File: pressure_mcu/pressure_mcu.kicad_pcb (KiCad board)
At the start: 2 copper layers, 33.2 x 35 mm, 41 parts, among them J2 USB_B_Micro, J4 1, J5 2, J6 3, J7 4, J8 SWD JST PH, U2 AP2112K-3.3, U4 STM32H562RGT6, U7 TCA9548APWR, Y2 12MHz

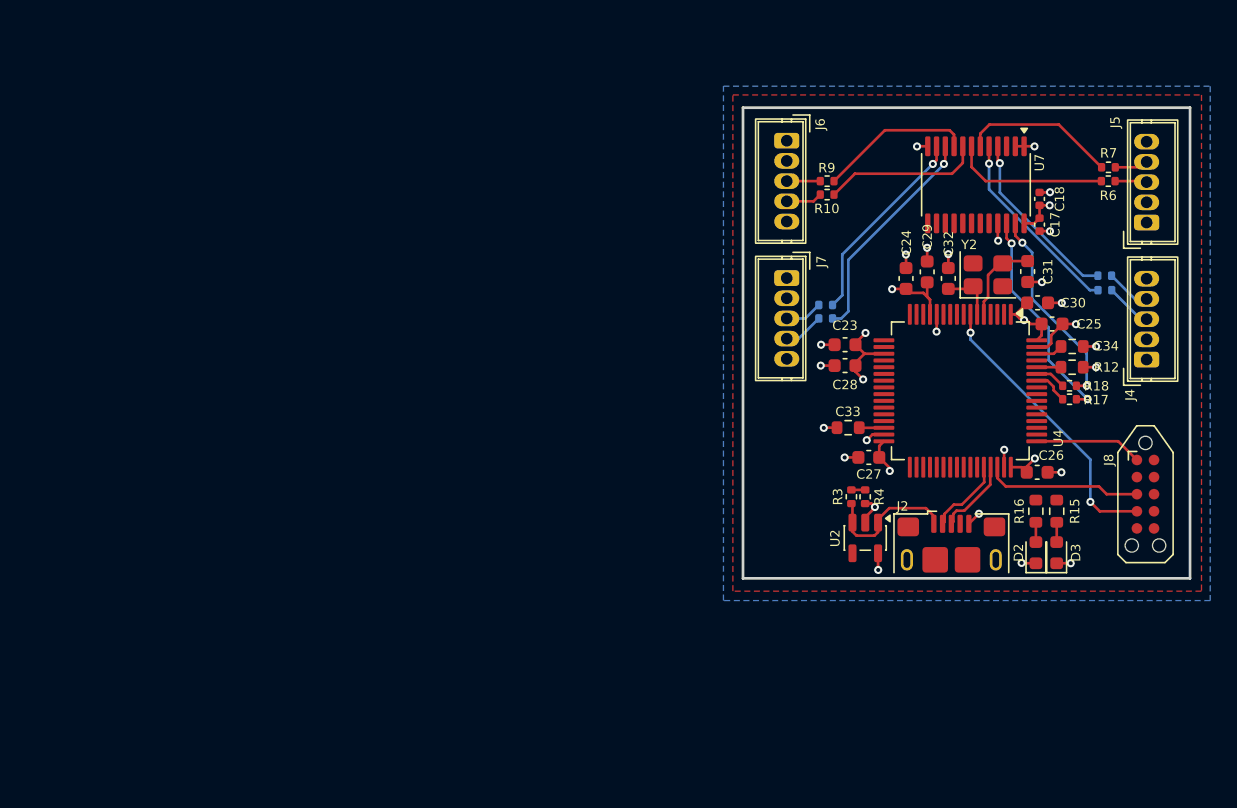
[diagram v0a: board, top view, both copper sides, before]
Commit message: ready for review
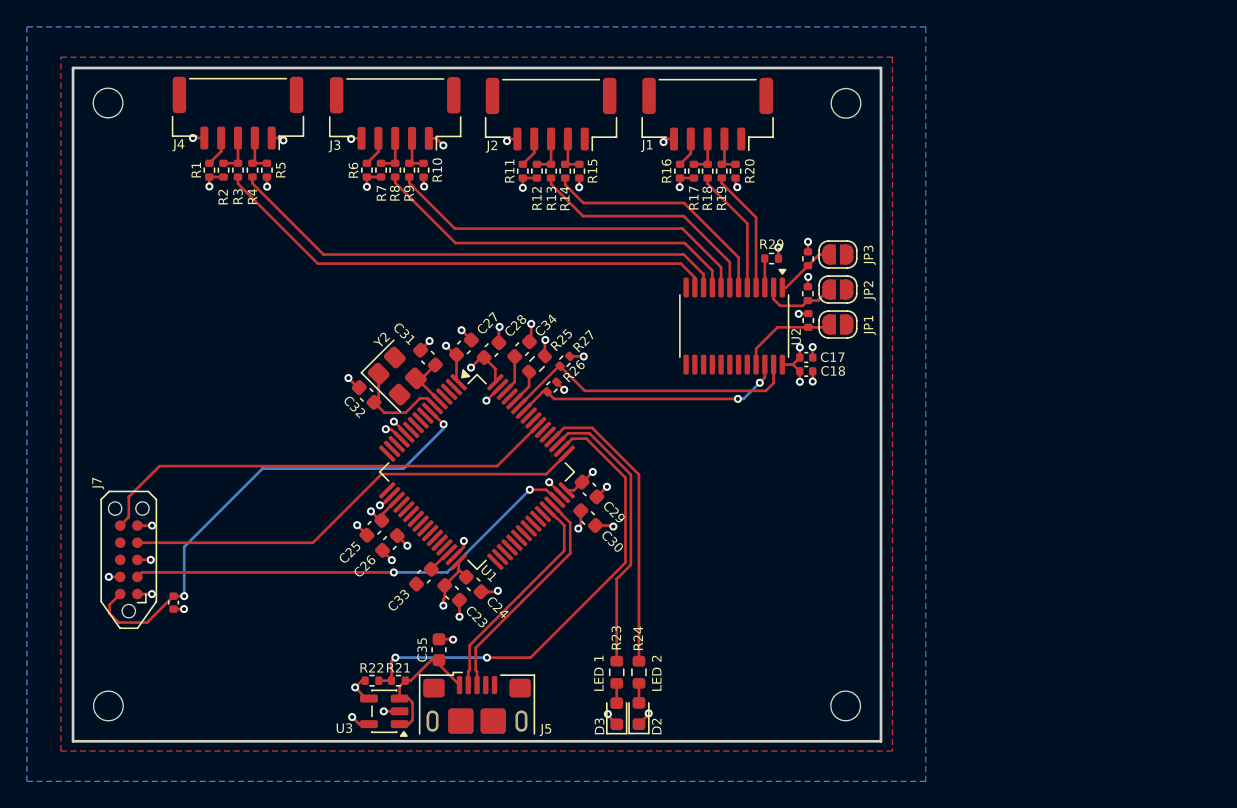
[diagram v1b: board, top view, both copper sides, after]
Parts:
- removed J6: 3, Connector_Wuerth:Wuerth_WR-WTB_64800511622_1x05_P1.50mm_Vertical
- removed J8: SWD JST PH, Connector:Tag-Connect_TC2050-IDC-NL_2x05_P1.27mm_Vertical_with_bottom_clip
- removed U4: STM32H562RGT6, Package_QFP:LQFP-64_10x10mm_P0.5mm
- removed U7: TCA9548APWR, Package_SO:TSSOP-24_4.4x7.8mm_P0.65mm
- added C35: 10uF, Capacitor_SMD:C_0603_1608Metric, F.Cu at (147.2, 118.2)
- added C36: 100nF, Capacitor_SMD:C_0402_1005Metric, F.Cu at (127.5, 114.7)
- added H1: MountingHole, MountingHole:MountingHole_2.2mm_M2, F.Cu at (122.6, 77.6)
- added H2: MountingHole, MountingHole:MountingHole_2.2mm_M2, F.Cu at (177.4, 77.6)
- added H3: MountingHole, MountingHole:MountingHole_2.2mm_M2, F.Cu at (122.6, 122.4)
- added H4: MountingHole, MountingHole:MountingHole_2.2mm_M2, F.Cu at (177.4, 122.4)
- added J1: 1, Connector_JST:JST_GH_SM05B-GHS-TB_1x05-1MP_P1.25mm_Horizontal, F.Cu at (167.1, 78.4)
- added J3: 3, Connector_JST:JST_GH_SM05B-GHS-TB_1x05-1MP_P1.25mm_Horizontal, F.Cu at (143.9, 78.4)
- added JP1: SolderJumper_2_Open, Jumper:SolderJumper-2_P1.3mm_Open_RoundedPad1.0x1.5mm, F.Cu at (176.8, 94.0)
- added JP2: SolderJumper_2_Open, Jumper:SolderJumper-2_P1.3mm_Open_RoundedPad1.0x1.5mm, F.Cu at (176.8, 91.5)
- added JP3: SolderJumper_2_Open, Jumper:SolderJumper-2_P1.3mm_Open_RoundedPad1.0x1.5mm, F.Cu at (176.8, 88.8)
- added R1: 10k, Resistor_SMD:R_0402_1005Metric, F.Cu at (130.1, 82.6)
- added R14: 0, Resistor_SMD:R_0402_1005Metric, F.Cu at (156.6, 82.7)
- added R19: 0, Resistor_SMD:R_0402_1005Metric, F.Cu at (168.2, 82.7)
- added R2: 2.2k, Resistor_SMD:R_0402_1005Metric, F.Cu at (131.2, 82.6)
- added R20: 2.2k, Resistor_SMD:R_0402_1005Metric, F.Cu at (169.2, 82.7)
- added R21: 10k, Resistor_SMD:R_0402_1005Metric, F.Cu at (144.2, 120.5)
- added R22: 15k, Resistor_SMD:R_0402_1005Metric, F.Cu at (142.2, 120.5)
- added R23: 220R, Resistor_SMD:R_0603_1608Metric, F.Cu at (160.4, 119.9)
- added R24: 220R, Resistor_SMD:R_0603_1608Metric, F.Cu at (162.0, 119.9)
- added R25: 10k, Resistor_SMD:R_0603_1608Metric, F.Cu at (154.4, 97.0)
- added R26: 2.2k, Resistor_SMD:R_0402_1005Metric, F.Cu at (155.6, 98.7)
- added R27: 2.2k, Resistor_SMD:R_0402_1005Metric, F.Cu at (156.5, 96.8)
- added R29: 10k, Resistor_SMD:R_0402_1005Metric, F.Cu at (171.9, 89.2)
- added R30: 10k, Resistor_SMD:R_0402_1005Metric, F.Cu at (174.6, 89.2)
- added R31: 10k, Resistor_SMD:R_0402_1005Metric, F.Cu at (174.6, 91.8)
- added R32: 10k, Resistor_SMD:R_0402_1005Metric, F.Cu at (174.6, 93.8)
- added U1: STM32H562RGT6, Package_QFP:LQFP-64_10x10mm_P0.5mm, F.Cu at (150.0, 105.0)
- added U3: AP2112K-3.3, Package_TO_SOT_SMD:SOT-23-5, F.Cu at (143.1, 122.8)
- C17: value 4u7F -> 4.7uF
- C31, C32: value 27pF -> 33pF
- C33, C34: value 2u2 -> 2.2uF; footprint Resistor_SMD:R_0603_1608Metric -> Capacitor_SMD:C_0603_1608Metric
- J2: value USB_B_Micro -> 2; footprint Connector_USB:USB_Micro-B_Amphenol_10118193-0001LF_Horizontal -> Connector_JST:JST_GH_SM05B-GHS-TB_1x05-1MP_P1.25mm_Horizontal
- J4: value 1 -> 4; footprint Connector_Wuerth:Wuerth_WR-WTB_64800511622_1x05_P1.50mm_Vertical -> Connector_JST:JST_GH_SM05B-GHS-TB_1x05-1MP_P1.25mm_Horizontal
- J5: value 2 -> USB_B_Micro; footprint Connector_Wuerth:Wuerth_WR-WTB_64800511622_1x05_P1.50mm_Vertical -> Connector_USB:USB_Micro-B_Amphenol_10118193-0001LF_Horizontal
- J7: value 4 -> SWD JST PH; footprint Connector_Wuerth:Wuerth_WR-WTB_64800511622_1x05_P1.50mm_Vertical -> Connector:Tag-Connect_TC2050-IDC-NL_2x05_P1.27mm_Vertical_with_bottom_clip
- R10, R7: value R -> 2.2k
- R11: value R -> 10k; moved to F.Cu
- R12: value 10k -> 2.2k; footprint Resistor_SMD:R_0603_1608Metric -> Resistor_SMD:R_0402_1005Metric
- R13, R8: value R -> 0; moved to F.Cu
- R15: value 220R -> 2.2k; footprint Resistor_SMD:R_0603_1608Metric -> Resistor_SMD:R_0402_1005Metric
- R16: value 220R -> 10k; footprint Resistor_SMD:R_0603_1608Metric -> Resistor_SMD:R_0402_1005Metric
- R18: value 2.2k -> 0
- R3: value 10k -> 0
- R4: value 15k -> 0
- R5: value R -> 2.2k; moved to F.Cu
- R6: value R -> 10k
- R9: value R -> 0
- U2: value AP2112K-3.3 -> TCA9548APWR; footprint Package_TO_SOT_SMD:SOT-23-5 -> Package_SO:TSSOP-24_4.4x7.8mm_P0.65mm
- moved J4 69.9 mm to (132.2, 78.3), turned to 180 degrees
- moved R5 62.7 mm to (134.4, 82.6), turned to 90 degrees
- moved J5 62.0 mm to (150.0, 123.5), turned to 0 degrees
- moved R6 55.1 mm to (141.8, 82.6), turned to 90 degrees
- moved R7 54.0 mm to (142.9, 82.6), turned to 90 degrees
- moved R8 53.4 mm to (143.9, 82.6), turned to 90 degrees
- moved J7 53.2 mm to (124.1, 111.5), turned to 90 degrees
- moved C25 52.6 mm to (142.4, 109.1), turned to -135 degrees
- moved R3 51.6 mm to (132.2, 82.6)
- moved R4 51.6 mm to (133.3, 82.6), turned to 90 degrees
- moved C26 48.4 mm to (143.5, 110.3), turned to -135 degrees
- moved C31 45.0 mm to (146.4, 96.5), turned to -45 degrees
- moved Y2 44.5 mm to (144.1, 97.9), turned to -45 degrees
- moved J2 44.5 mm to (155.5, 78.4), turned to 180 degrees
- moved C32 44.1 mm to (141.8, 99.3), turned to 135 degrees
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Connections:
- J2 pad 1: /V_BUS -> GND
- J2 pad 2: /USB_D- -> /MUX1_SDA
- J2 pad 3: /USB_D+ -> /MUX1_SCL
- J2 pad 4: unconnected-(J2-ID-Pad4) -> /MUX1_NRST
- J2 pad 5: GND -> +3V3
- J4 pad 1: +3V3 -> GND
- J4 pad 2: /MUX2_NRST -> /MUX4_SDA
- J4 pad 3: /MUX2_SCL -> /MUX4_SCL
- J4 pad 4: /MUX2_SDA -> /MUX4_NRST
- J4 pad 5: GND -> +3V3
- J5 pad 1: +3V3 -> /V_BUS
- J5 pad 2: /MUX1_NRST -> /USB_D-
- J5 pad 3: /MUX1_SCL -> /USB_D+
- J5 pad 4: /MUX1_SDA -> unconnected-(J5-ID-Pad4)
- J7 pad 2: /MUX4_NRST -> /SWDIO
- J7 pad 3: /MUX4_SCL -> GND
- J7 pad 4: /MUX4_SDA -> /SWCLK
- R10 pad 1: Net-(U7-SD2) -> +3V3
- R11 pad 1: Net-(U7-SC3) -> +3V3
- R11 pad 2: /MUX4_SCL -> /MUX1_NRST
- R12 pad 1: Net-(U4-BOOT0) -> +3V3
- R12 pad 2: GND -> /MUX1_SCL
- R13 pad 1: Net-(U7-SD3) -> Net-(U2-SC1)
- R13 pad 2: /MUX4_SDA -> /MUX1_SCL
- R15 pad 1: /LED1 -> +3V3
- R15 pad 2: Net-(D3-A) -> /MUX1_SDA
- R16 pad 1: /LED2 -> +3V3
- R16 pad 2: Net-(D2-A) -> /MUX2_NRST
- R17 pad 1: Net-(U7-SCL) -> +3V3
- R17 pad 2: /MUX_SCL -> /MUX2_SCL
- R18 pad 1: Net-(U7-SDA) -> Net-(U2-SC0)
- R18 pad 2: /MUX_SDA -> /MUX2_SCL
- R3 pad 1: /V_BUS -> Net-(U2-SC3)
- R3 pad 2: /V_SENSE -> /MUX4_SCL
- R4 pad 1: /V_SENSE -> Net-(U2-SD3)
- R4 pad 2: GND -> /MUX4_SDA
- R5 pad 1: Net-(U7-SD0) -> +3V3
- R5 pad 2: /MUX2_SDA -> /MUX4_SDA
- R6 pad 1: Net-(U7-SC1) -> +3V3
- R6 pad 2: /MUX1_SCL -> /MUX3_NRST
- R7 pad 1: Net-(U7-SD1) -> +3V3
- R7 pad 2: /MUX1_SDA -> /MUX3_SCL
- R8 pad 1: Net-(U7-SC0) -> Net-(U2-SC2)
- R8 pad 2: /MUX2_SCL -> /MUX3_SCL
- R9 pad 1: Net-(U7-SC2) -> Net-(U2-SD2)
- R9 pad 2: /MUX3_SCL -> /MUX3_SDA
- U2 pad 1: /V_BUS -> /A0
- U2 pad 2: GND -> /A1
- U2 pad 3: /V_BUS -> /MUX_NRST
- U2 pad 4: unconnected-(U2-NC-Pad4) -> Net-(U2-SD0)
- U2 pad 5: +3V3 -> Net-(U2-SC0)
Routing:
- net Net-(U2-SC3): track 0.00 -> 38.1 mm
- net Net-(U2-SD3): track 0.00 -> 37.8 mm
- net /nRESET: track 0.00 -> 36.7 mm, vias 0 -> 2
- net /SWO: track 0.00 -> 35.0 mm
- net /V_SENSE: track 1.02 -> 35.3 mm, vias 0 -> 2
- net Net-(U2-SC2): track 0.00 -> 27.9 mm
- net Net-(U2-SD2): track 0.00 -> 27.7 mm
- net /SWCLK: track 8.02 -> 34.6 mm
- net /SWDIO: track 11.7 -> 34.2 mm, vias 0 -> 2
- net /LED2: track 0.00 -> 22.1 mm
- net /NRST: track 21.4 -> 0.00 mm, vias 2 -> 0
- net /LED1: track 0.00 -> 21.4 mm
- net /MUX_SDA: track 2.29 -> 22.5 mm
- net +3V3: track 26.3 -> 45.1 mm, vias 8 -> 30
- net Net-(U2-SC1): track 0.00 -> 18.0 mm
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- added copper zone on In2.Cu, net +3V3
- added copper zone on B.Cu, net GND
- added copper zone on In1.Cu, net GND
- removed copper zone on B.Cu, net +3V3
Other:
- board size 33.2 x 35 mm -> 60 x 50 mm
- copper layers 2 -> 4
- board text added: "LED 1"
- board text added: "LED 2"
- board text added: "Pressure MCU"
- board text added: "REV A"
- board text added: "UCM 26"
